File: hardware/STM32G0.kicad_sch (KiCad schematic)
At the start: 17 parts, among them T1 TP_+3V3, U1 STM32G0C1KCTxN

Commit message: changed pcb layout
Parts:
- D1, D2, D3, D8: footprint LED_SMD:LED_01005_0402Metric_Pad0.57x0.30mm_HandSolder -> LED_SMD:LED_0603_1608Metric_Pad1.05x0.95mm_HandSolder
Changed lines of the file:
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@@
 			)
 		)
-		(property "Footprint" "LED_SMD:LED_01005_0402Metric_Pad0.57x0.30mm_HandSolder"
+		(property "Footprint" "LED_SMD:LED_0603_1608Metric_Pad1.05x0.95mm_HandSolder"
 			(at 85.09 116.84 90)
 			(hide yes)
@@
 			)
 		)
-		(property "Footprint" "LED_SMD:LED_01005_0402Metric_Pad0.57x0.30mm_HandSolder"
+		(property "Footprint" "LED_SMD:LED_0603_1608Metric_Pad1.05x0.95mm_HandSolder"
 			(at 85.09 137.16 90)
 			(hide yes)
@@
 			)
 		)
-		(property "Footprint" "LED_SMD:LED_01005_0402Metric_Pad0.57x0.30mm_HandSolder"
+		(property "Footprint" "LED_SMD:LED_0603_1608Metric_Pad1.05x0.95mm_HandSolder"
 			(at 85.09 142.24 90)
 			(hide yes)
@@
 			)
 		)
-		(property "Footprint" "LED_SMD:LED_01005_0402Metric_Pad0.57x0.30mm_HandSolder"
+		(property "Footprint" "LED_SMD:LED_0603_1608Metric_Pad1.05x0.95mm_HandSolder"
 			(at 85.09 127 90)
 			(hide yes)

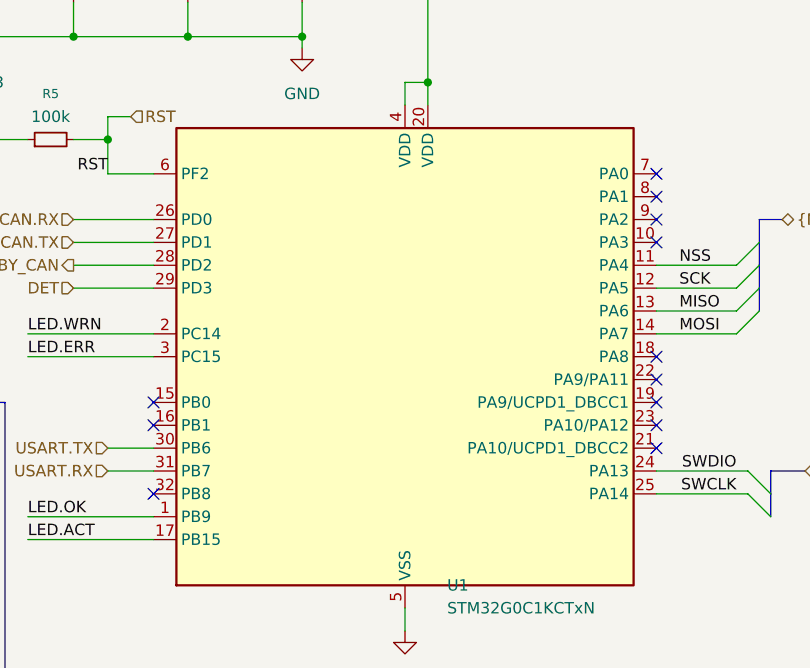
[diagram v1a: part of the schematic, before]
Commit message: fixed routing issues
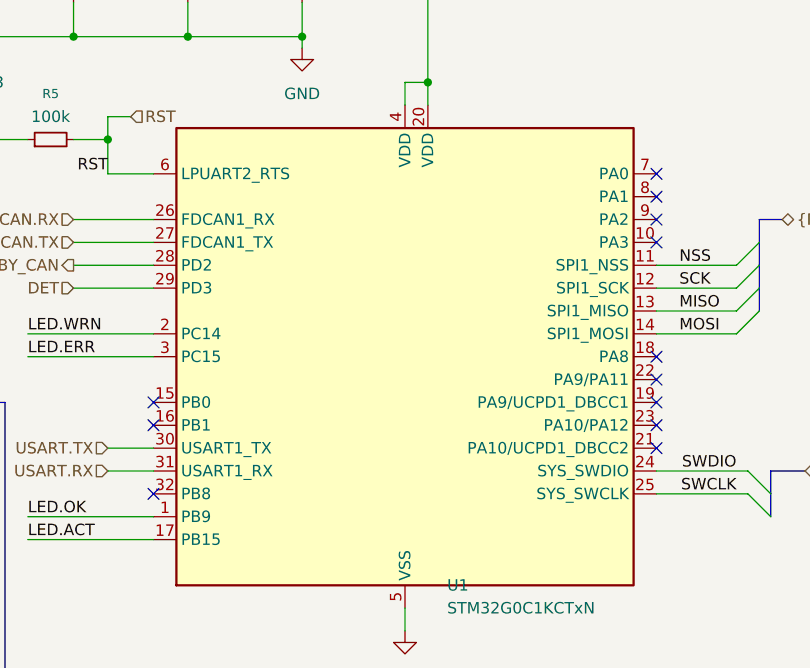
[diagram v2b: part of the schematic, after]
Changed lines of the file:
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@@
 		)
 		(pin "30"
+			(alternate "USART1_TX")
 		)
 		(pin "31"
+			(alternate "USART1_RX")
 		)
 		(pin "8"
 		)
 		(pin "14"
+			(alternate "SPI1_MOSI")
 		)
 		(pin "23"
@@
 		)
 		(pin "24"
+			(alternate "SYS_SWDIO")
 		)
 		(pin "13"
+			(alternate "SPI1_MISO")
 		)
 		(pin "5"
@@
 		)
 		(pin "11"
+			(alternate "SPI1_NSS")
 		)
 		(pin "32"
 		)
 		(pin "26"
+			(alternate "FDCAN1_RX")
 		)
 		(pin "16"
 		)
 		(pin "12"
+			(alternate "SPI1_SCK")
 		)
 		(pin "10"
 		)
 		(pin "6"
+			(alternate "LPUART2_RTS")
 		)
 		(pin "9"
@@
 		)
 		(pin "25"
+			(alternate "SYS_SWCLK")
 		)
 		(pin "27"
+			(alternate "FDCAN1_TX")
 		)
 		(pin "22"
